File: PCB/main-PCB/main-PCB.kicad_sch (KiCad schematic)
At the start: 25 parts, among them Q1 SSM6J214FE, Q2 Q_NMOS_GSD, U1 LIS2DU12TR, U2 STM32U031K4Ux

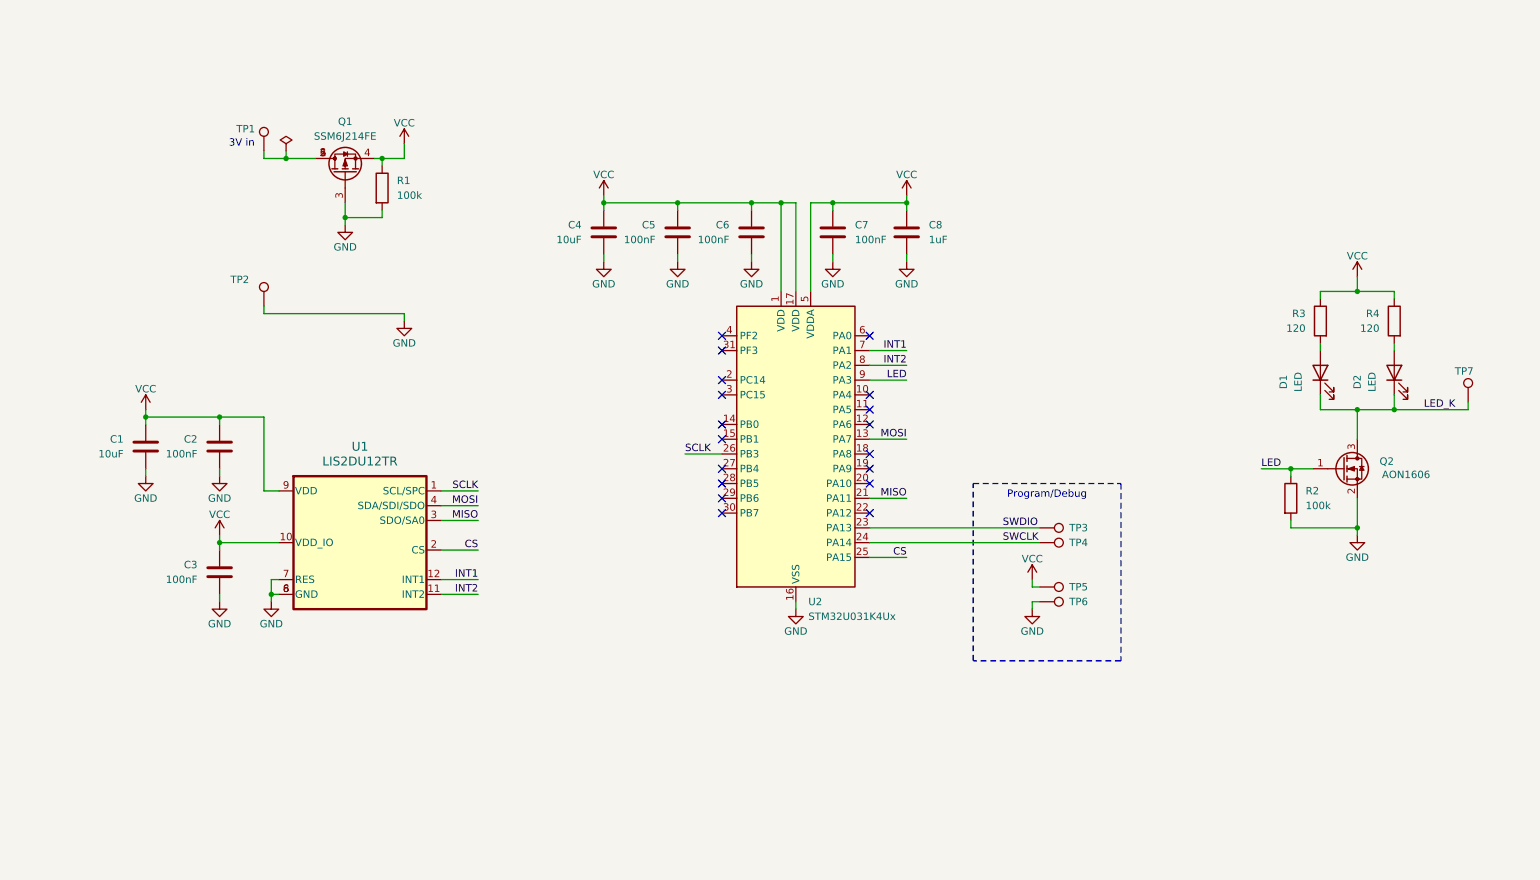
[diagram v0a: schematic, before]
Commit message: Updated PCB STEP file
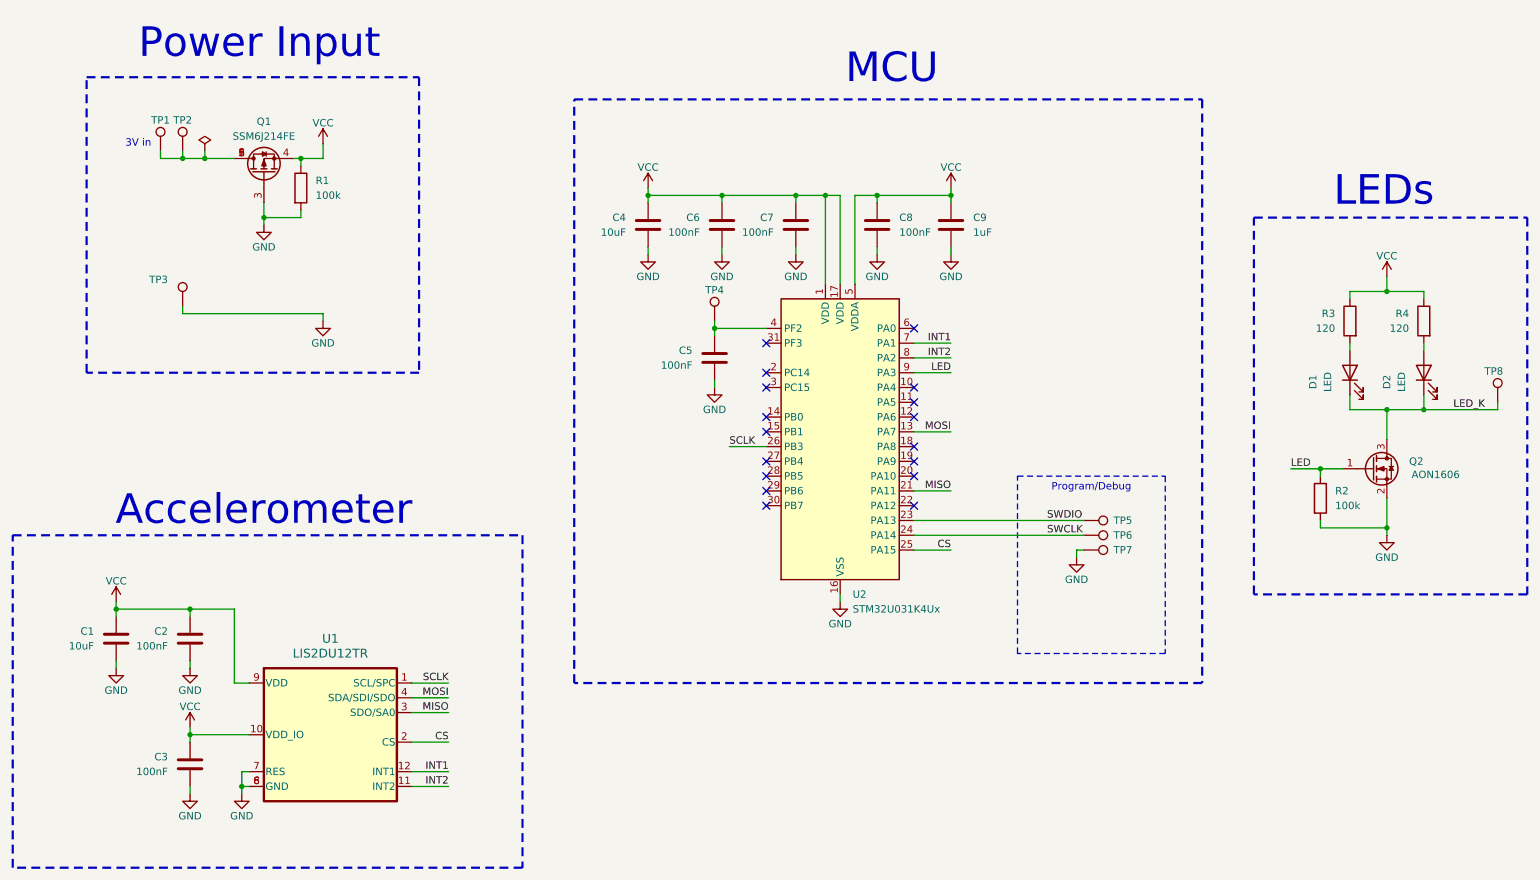
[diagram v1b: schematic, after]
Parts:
- removed TP5: TestPoint, TestPoint:TestPoint_Pad_D1.0mm, symbol Connector:TestPoint
- added C5: 100nF, Capacitor_SMD:C_0402_1005Metric, symbol Device:C
- added TP2: TestPoint, TestPoint:TestPoint_Pad_D1.0mm, symbol Connector:TestPoint
- added TP4: TestPoint, EN_Designs-Footprints:TestPoint_Pad_D0.5mm, symbol Connector:TestPoint
- TP5: renamed from TP3; now left out of the parts list
- TP6: renamed from TP4; now left out of the parts list
- TP7: renamed from TP6; now left out of the parts list
- U2: MPN (none) -> STM32U031K4U6
- renumbered C5 to C6, C6 to C7, C7 to C8, C8 to C9, TP2 to TP3, TP7 to TP8
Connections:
- net GND: now also C5.2
- net at Q1.1 (D), Q1.2 (D), Q1.5 (D)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: now also TP2.1
- net at U2.4 (PF2): now also C5.1, TP4.1
- no-connect marks 18 -> 17
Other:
- note added: "Accelerometer"
- note added: "LEDs"
- note added: "MCU"
- note added: "Power Input"
- moved on the sheet: C1, C2, C3, C4, C6, C7, C8, C9, D1, D2, Q1, Q2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
